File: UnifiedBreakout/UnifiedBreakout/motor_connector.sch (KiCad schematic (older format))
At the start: 1 part, among them J7 RJ45

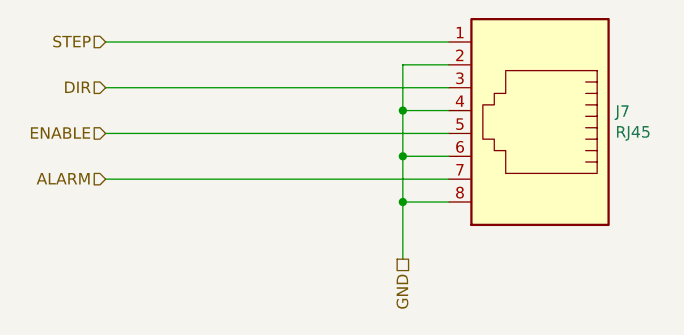
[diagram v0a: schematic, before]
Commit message: Finished(?) unified breakout layout
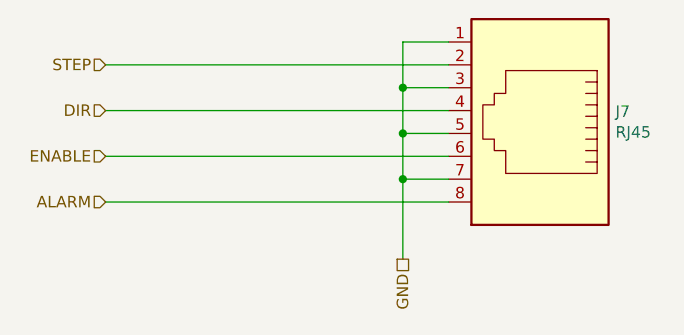
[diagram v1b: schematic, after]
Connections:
- net ALARM: now also J7.8; no longer J7.7
- net DIR: now also J7.4; no longer J7.3
- net ENABLE: now also J7.6; no longer J7.5
- net GND: now also J7.1, J7.3, J7.5, J7.7; no longer J7.2, J7.4, J7.6, J7.8
- net STEP: now also J7.2; no longer J7.1
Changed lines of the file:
@@
 $EndComp
 Wire Wire Line
-	5000 3150 4800 3150
+	5000 3150 3500 3150
 Wire Wire Line
-	4800 3150 4800 3350
+	5000 3350 3500 3350
 Wire Wire Line
-	5000 3350 4800 3350
-Connection ~ 4800 3350
-Wire Wire Line
-	4800 3350 4800 3550
-Wire Wire Line
-	5000 3550 4800 3550
-Connection ~ 4800 3550
-Wire Wire Line
-	4800 3550 4800 3750
-Wire Wire Line
-	5000 3750 4800 3750
-Connection ~ 4800 3750
-Wire Wire Line
-	5000 3050 3500 3050
-Wire Wire Line
-	5000 3250 3500 3250
-Wire Wire Line
-	5000 3450 3500 3450
-Wire Wire Line
-	5000 3650 3500 3650
-Wire Wire Line
-	4800 3750 4800 4000
-Text HLabel 3500 3050 0    50   Input ~ 0
+	5000 3750 3500 3750
+Text HLabel 3500 3150 0    50   Input ~ 0
 STEP
-Text HLabel 3500 3250 0    50   Input ~ 0
+Text HLabel 3500 3350 0    50   Input ~ 0
 DIR
-Text HLabel 3500 3450 0    50   Input ~ 0
+Text HLabel 3500 3550 0    50   Input ~ 0
 ENABLE
-Text HLabel 3500 3650 0    50   Input ~ 0
+Text HLabel 3500 3750 0    50   Input ~ 0
 ALARM
 Text HLabel 4800 4000 3    50   UnSpc ~ 0
 GND
+Wire Wire Line
+	5000 3550 3500 3550
+Wire Wire Line
+	5000 3050 4800 3050
+Wire Wire Line
+	4800 3050 4800 3250
+Wire Wire Line
+	5000 3250 4800 3250
+Connection ~ 4800 3250
+Wire Wire Line
+	4800 3250 4800 3450
+Wire Wire Line
+	5000 3450 4800 3450
+Connection ~ 4800 3450
+Wire Wire Line
+	4800 3450 4800 3650
+Wire Wire Line
+	5000 3650 4800 3650
+Connection ~ 4800 3650
+Wire Wire Line
+	4800 3650 4800 4000
 $EndSCHEMATC

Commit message: Updated BOM
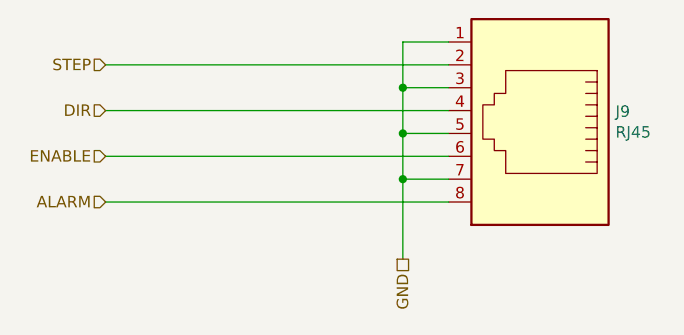
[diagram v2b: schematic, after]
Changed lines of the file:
@@
 AR Path="/5E67FD54/5E675BA7" Ref="J8"  Part="1"
 AR Path="/5E67FFE4/5E675BA7" Ref="J9"  Part="1"
-F 0 "J7" H 5070 3354 50  0000 R CNN
+F 0 "J9" H 5070 3354 50  0000 R CNN
 F 1 "RJ45" H 5070 3445 50  0000 R CNN
 F 2 "Stewart:SS6488SANF1" V 5400 3375 50  0001 C CNN

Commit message: Final updates to unified BoB
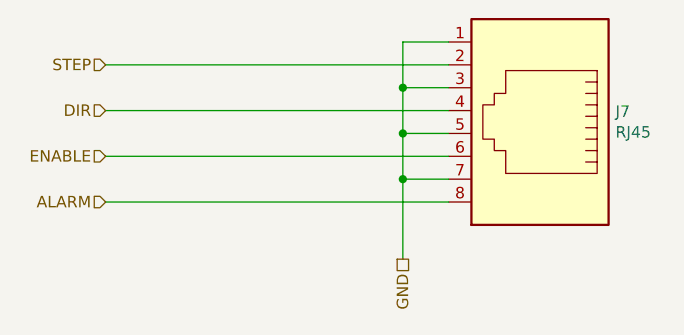
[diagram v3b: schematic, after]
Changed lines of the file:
@@
 AR Path="/5E67FD54/5E675BA7" Ref="J8"  Part="1"
 AR Path="/5E67FFE4/5E675BA7" Ref="J9"  Part="1"
-F 0 "J9" H 5070 3354 50  0000 R CNN
+F 0 "J7" H 5070 3354 50  0000 R CNN
 F 1 "RJ45" H 5070 3445 50  0000 R CNN
 F 2 "Stewart:SS6488SANF1" V 5400 3375 50  0001 C CNN
